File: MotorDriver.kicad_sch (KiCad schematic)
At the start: 24 parts, among them J1 43045-0402, Q1 NVMFD5C672NLT1G, Q2 NVMFD5C672NLT1G, Q3 NVMFD5C672NLT1G, Q4 NVMFD5C672NLT1G, U1 DRV8711DCP

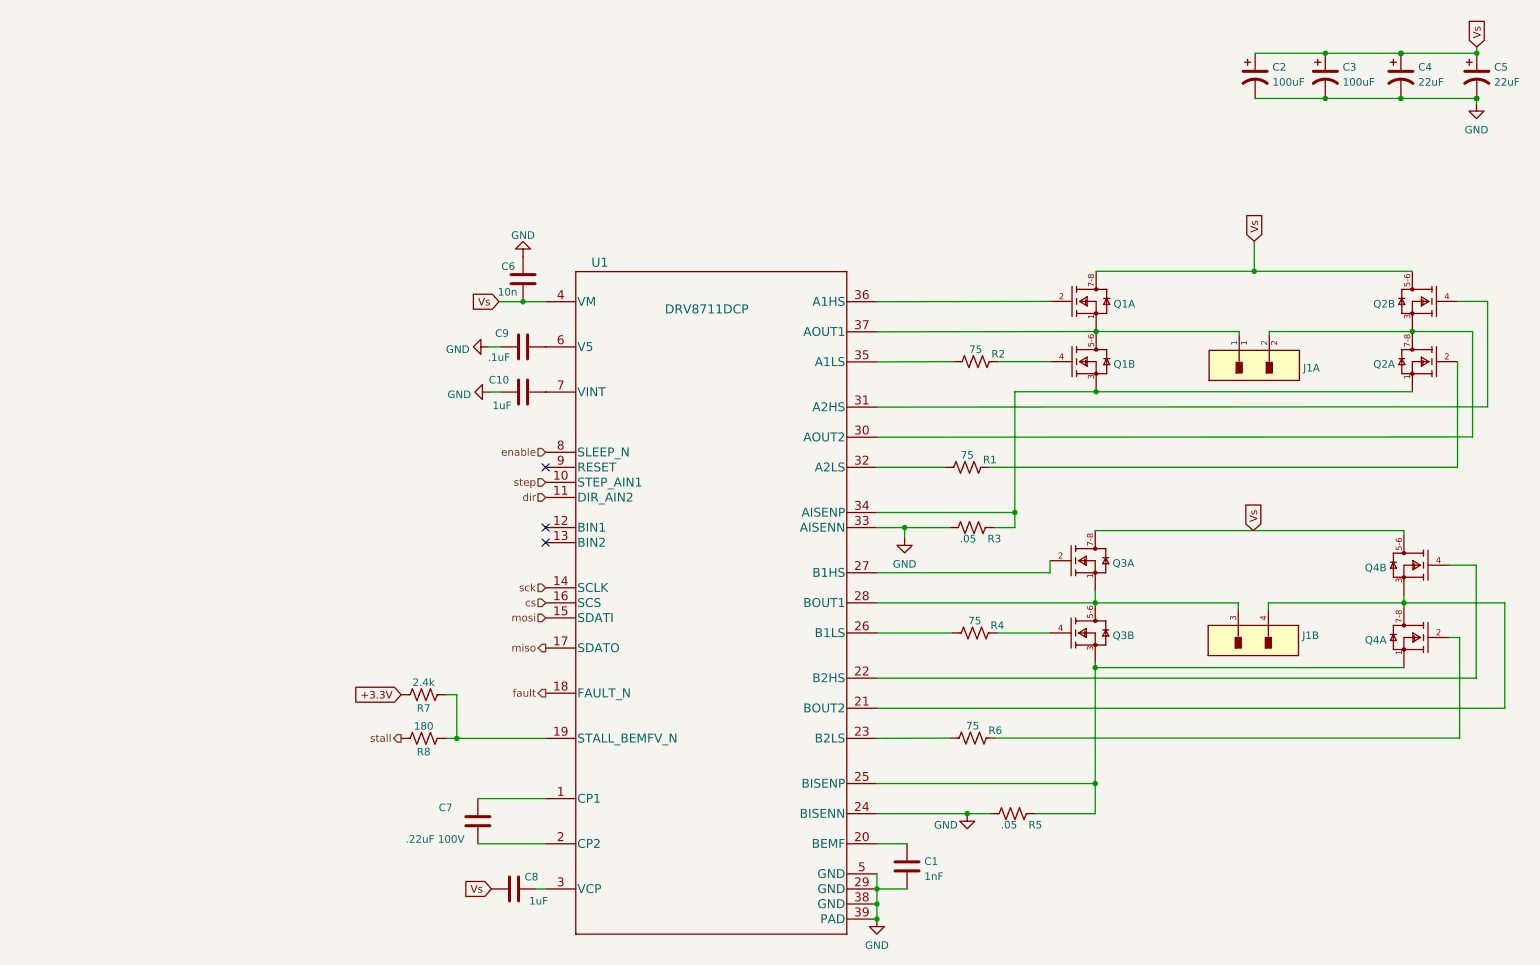
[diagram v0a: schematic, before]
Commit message: put all schematics on 50 mil grid
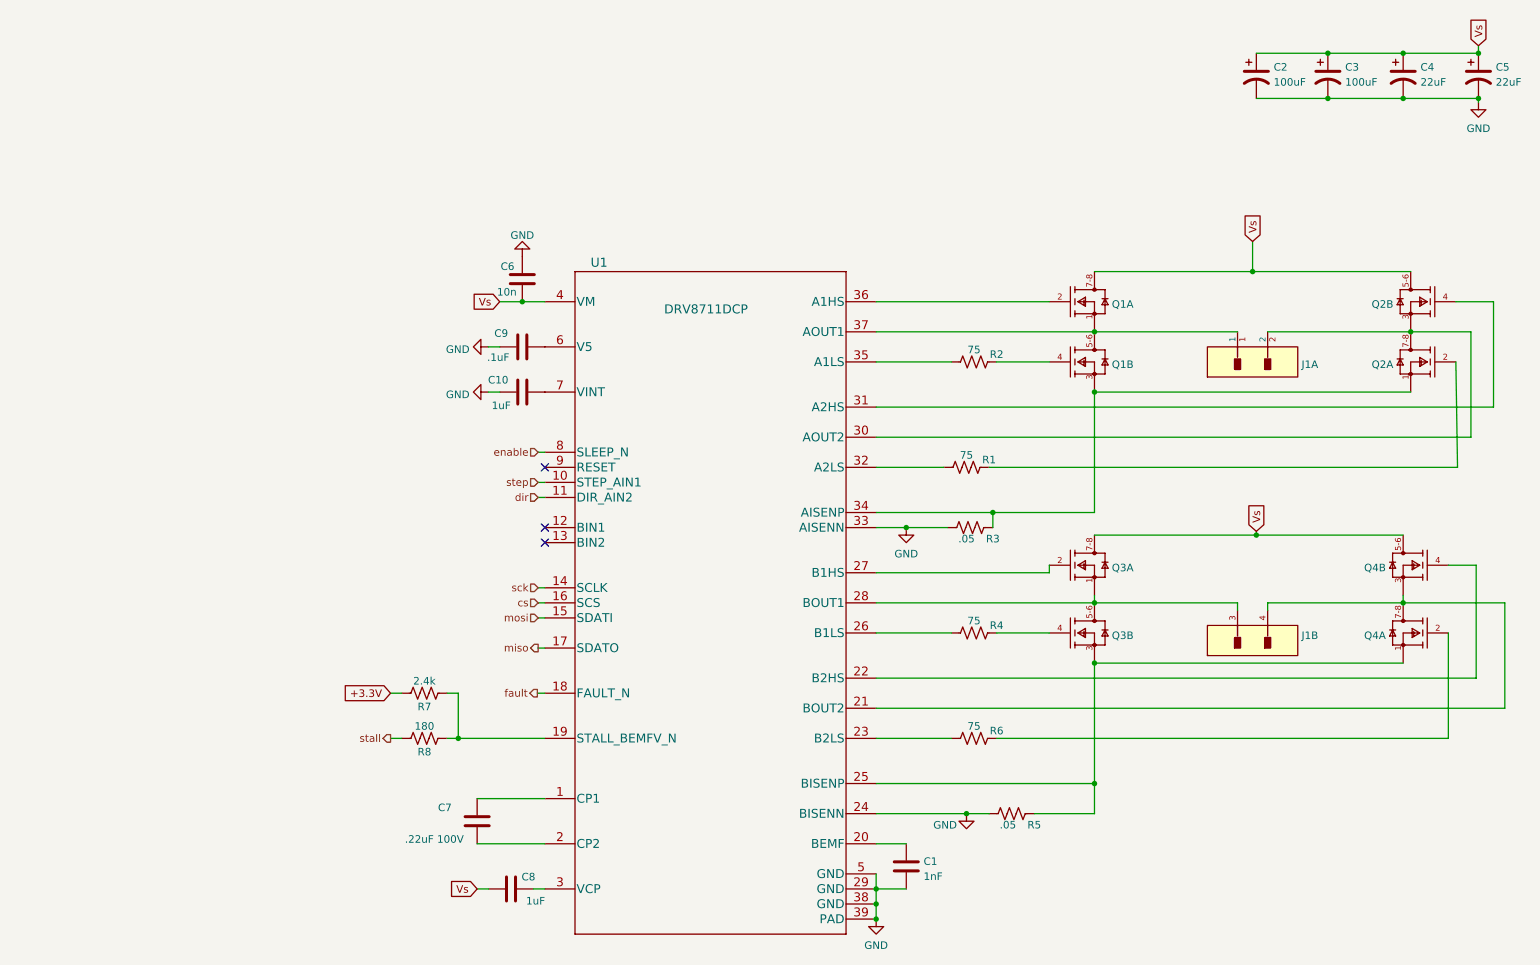
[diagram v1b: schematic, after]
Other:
- moved on the sheet: C8, J1A, Q3A, Q4A

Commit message: first commit of V18
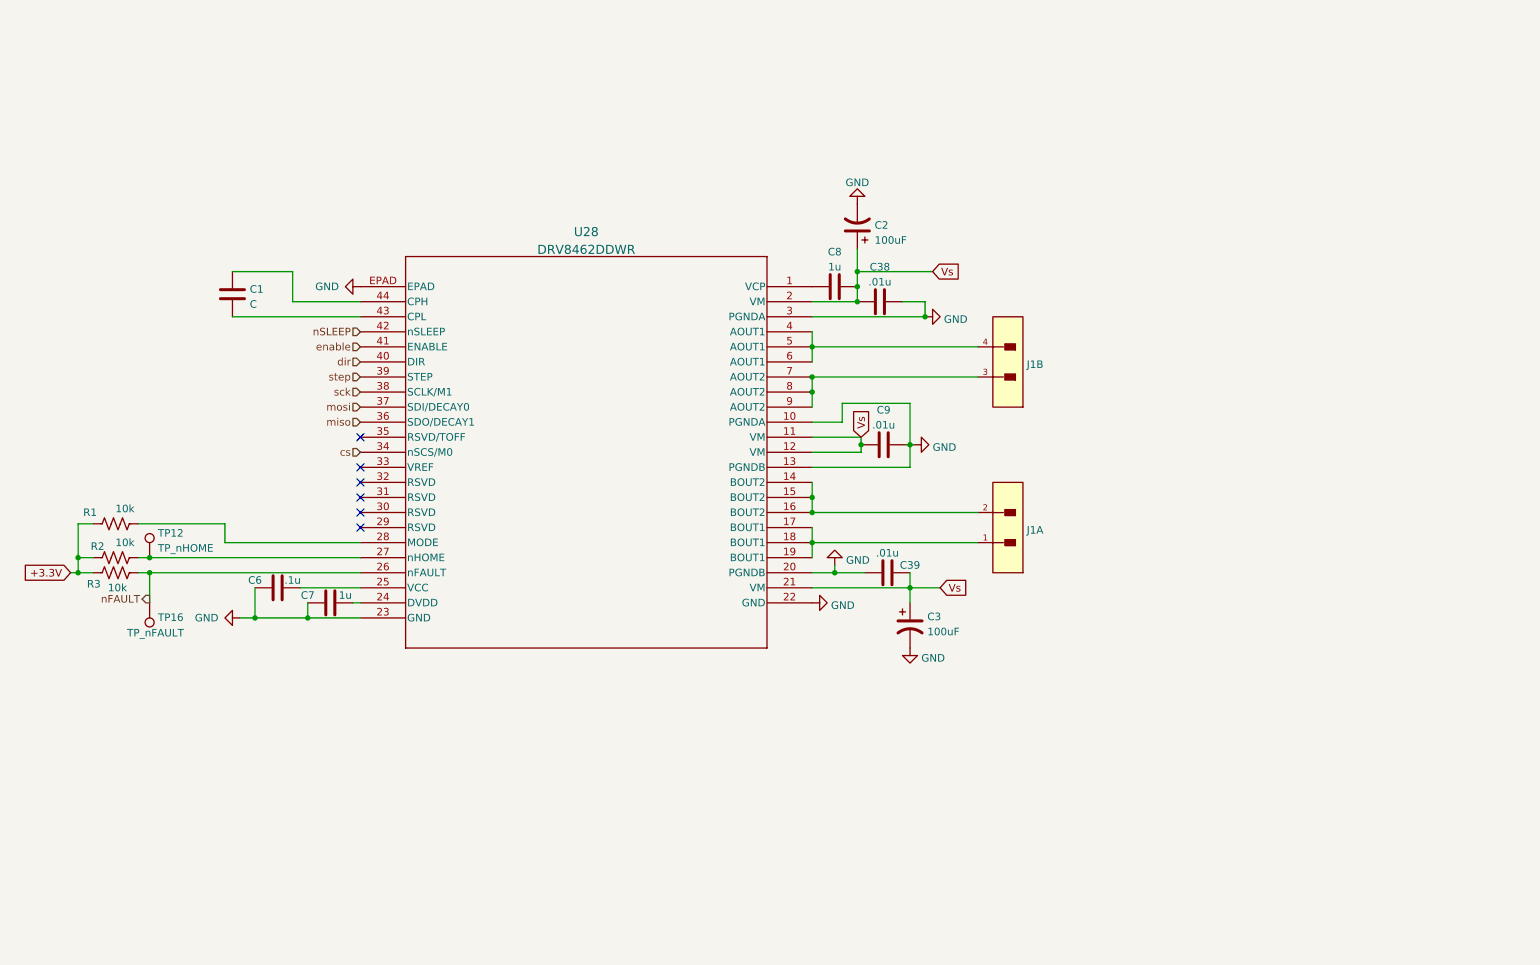
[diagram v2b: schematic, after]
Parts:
- removed C10: 1uF, Capacitor_SMD:C_0805_2012Metric_Pad1.18x1.45mm_HandSolder, symbol Device:C
- removed C4, C5: 22uF, Capacitor_THT:CP_Radial_D5.0mm_P2.00mm, symbol Device:C_Polarized_US
- removed Q1, Q2, Q3, Q4: NVMFD5C672NLT1G, Project_Footprints_Library:ON_Semiconductor-506BT-02_2013-E-MFG, symbol 1LibBBCTRL:NVMFD5C672NLT1G
- removed R4, R6: 75, Resistor_SMD:R_0805_2012Metric_Pad1.20x1.40mm_HandSolder, symbol Device:R_US
- removed R5: .05, Resistor_SMD:R_2512_6332Metric_Pad1.40x3.35mm_HandSolder, symbol Device:R_US
- removed R7: 2.4k, Resistor_SMD:R_0805_2012Metric_Pad1.20x1.40mm_HandSolder, symbol Device:R_US
- removed R8: 180, Resistor_SMD:R_0805_2012Metric_Pad1.20x1.40mm_HandSolder, symbol Device:R_US
- removed U1: DRV8711DCP, Project_Footprints_Library:DRV8711DCP, symbol 1LibBBCTRL:DRV8711DCP
- added C38, C39: .01u, Capacitor_SMD:C_0805_2012Metric_Pad1.18x1.45mm_HandSolder, symbol Device:C
- added TP12: TP_nHOME, Project_Footprints_Library:test_point, symbol Connector:TestPoint
- added TP16: TP_nFAULT, Project_Footprints_Library:test_point, symbol Connector:TestPoint
- added U28: DRV8462DDWR, Project_Footprints_Library:DDW44_8P26X4P31, symbol 1LibBBCTRL:DRV8462DDWR
- C1: value 1nF -> C; Model C0805C102K4RACTU -> CL21B104KCFNNNE
- C6: value 10n -> .1u; Model C0805C103K1RAC7210 -> 08056D104KAT2A
- C7: value .22uF 100V -> 1u; Model CL21B224KCFSNWE -> CC0805KKX5R5BB105
- C8: value 1uF -> 1u; Model CC0805KKX7R7BB105 -> CL05A104KA5NNNC
- C9: value .1uF -> .01u; Model C0805C104M5RACTU -> CAP CER 10000PF 100V X7R 0805
- R1, R2: value 75 -> 10k; Model RMCF0805JT75R0 -> RC0805FR-0710KL
- R3: value .05 -> 10k; footprint Resistor_SMD:R_2512_6332Metric_Pad1.40x3.35mm_HandSolder -> Resistor_SMD:R_0805_2012Metric_Pad1.20x1.40mm_HandSolder; Model CSRL3-0R05F8 -> RC0805FR-0710KL
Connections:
- net +3.3V: now also R1.1, R2.1, R3.1
- net GND: now also C7.1, C9.2, C38.2, C39.1, U28.10 (PGNDA), U28.13 (PGNDB), U28.20 (PGNDB), U28.22 (GND), U28.23 (GND), U28.3 (PGNDA), U28.EPAD; no longer C1.2, C9.1, R3.1
- net Vs: now also C8.1, C9.1, C38.1, C39.2, U28.11 (VM), U28.12 (VM), U28.2 (VM), U28.21 (VM); no longer C6.2, C8.2
- net cs: now also U28.34 (nSCS/M0)
- net dir: now also U28.40 (DIR)
- net enable: now also U28.41 (ENABLE)
- net miso: now also U28.36 (SDO/DECAY1)
- net mosi: now also U28.37 (SDI/DECAY0)
- net sck: now also U28.38 (SCLK/M1)
- net step: now also U28.39 (STEP)
- net at C7.2: now also U28.24 (DVDD)
- net at C1.1: now also U28.44 (CPH)
- net at J1.2: now also U28.14 (BOUT2), U28.15 (BOUT2), U28.16 (BOUT2)
- net at R2.2: now also TP12.1, U28.27 (nHOME)
- net nFAULT: now reaches R3.2
- net nFAULT: now also TP16.1, U28.26 (nFAULT)
- net at J1.1: now also U28.17 (BOUT1), U28.18 (BOUT1), U28.19 (BOUT1)
- net at R1.2: now also U28.28 (MODE)
- net at J1.3: now also U28.7 (AOUT2), U28.8 (AOUT2), U28.9 (AOUT2)
- net at J1.4: now also U28.4 (AOUT1), U28.5 (AOUT1), U28.6 (AOUT1)
- new net: C6.2, U28.25 (VCC)
- new net: C8.2, U28.1 (VCP)
- new net: C1.2, U28.43 (CPL)
- new net nSLEEP: U28.42 (nSLEEP)
- no-connect marks 3 -> 6
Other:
- moved on the sheet: C2, C3, J1B
